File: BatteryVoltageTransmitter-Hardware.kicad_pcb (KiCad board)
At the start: 2 copper layers, 51.8 x 54.4 mm, 5 parts, among them U1 MSP_EXP432P401R_Launchpad_Shi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, U2 Raspberry_Pi

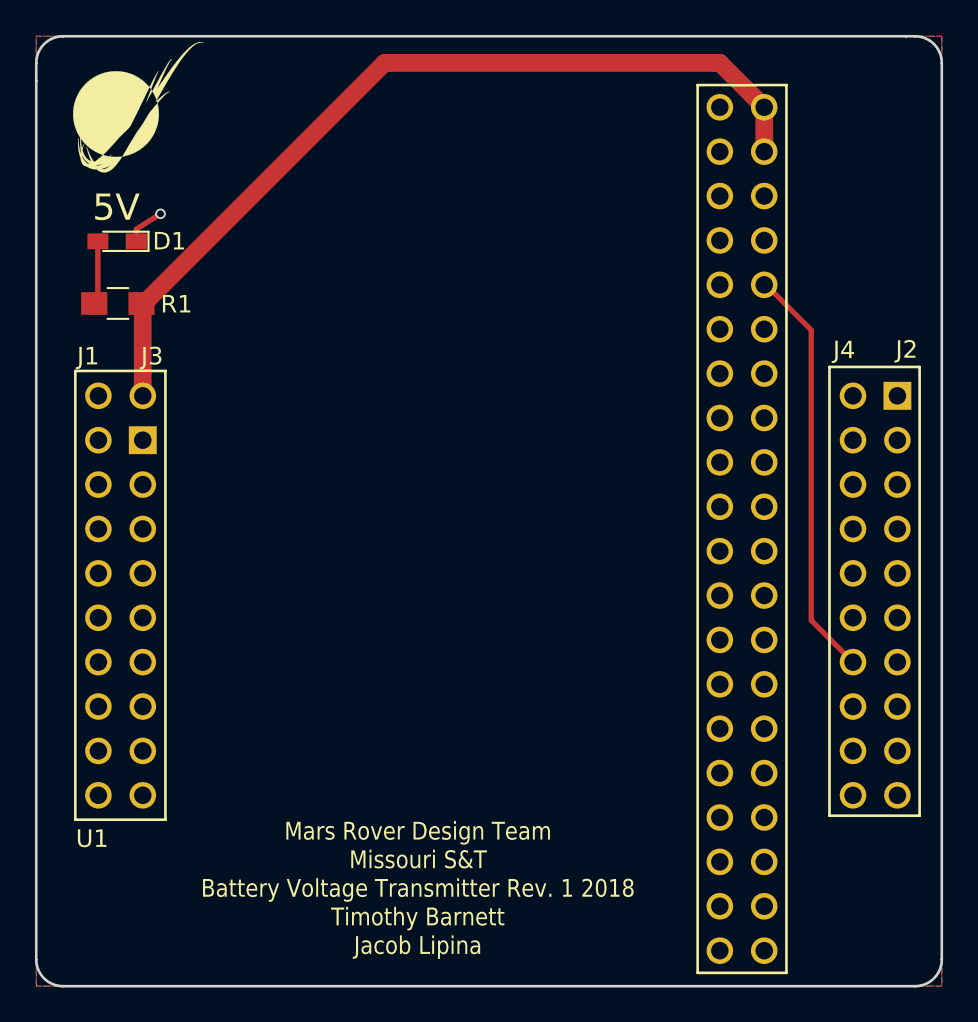
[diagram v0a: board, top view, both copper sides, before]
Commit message: Logos updated
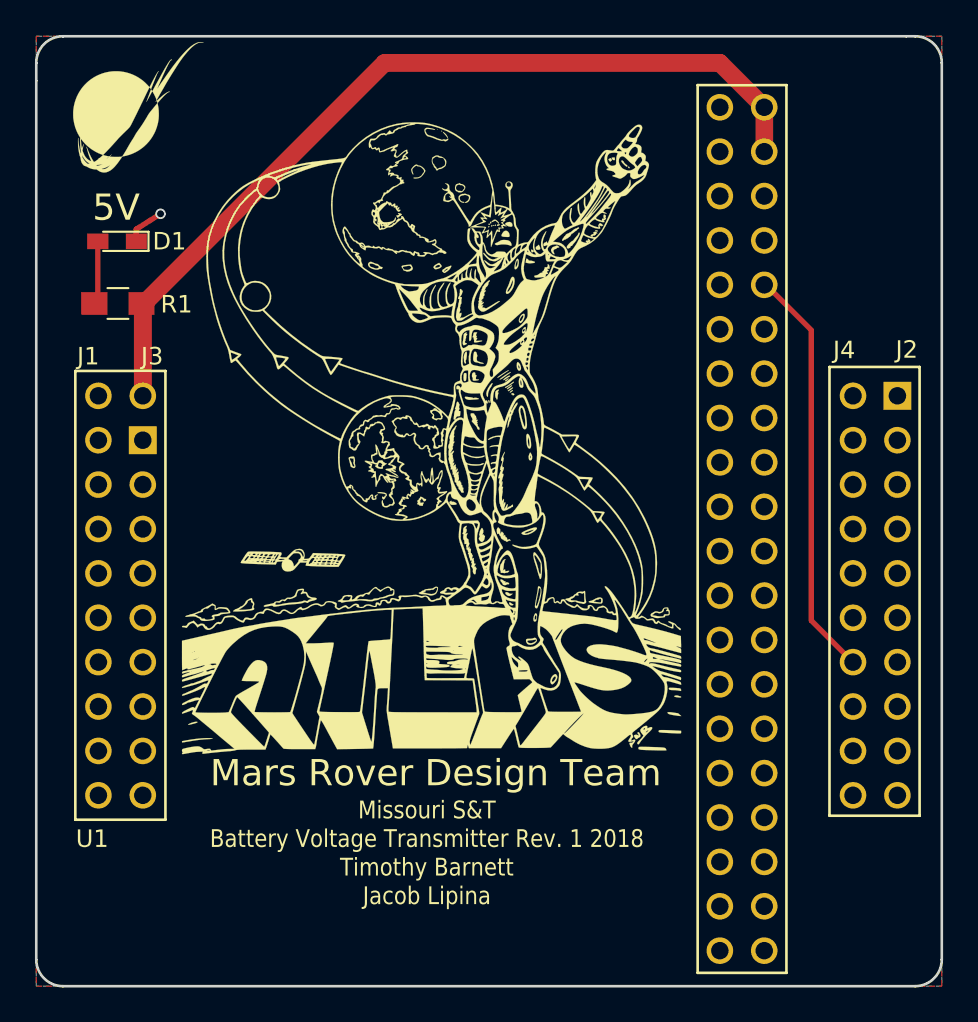
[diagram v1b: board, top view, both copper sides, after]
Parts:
- added S2: Logo_or_Signature, MRDT-Silkscreens:Atlas_Logo_28.6mmX37.3mm, F.Cu at (148.6, 82.0)
- S1: value MRDT_Logo -> Logo_or_Signature
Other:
- board text added: "Mars Rover Design Team"
- board text added: "Missouri S&T Battery Voltage Transmitter Rev. 1 2018 Timothy Barnett Jacob Lipina"
- board text removed: "Mars Rover Design Team Missouri S&T Battery Voltage Transmitter Rev. 1 2018 Timothy Barnett Jacob Lipina"
